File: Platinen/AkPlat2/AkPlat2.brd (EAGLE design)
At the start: 61.8 x 50.4 mm, 16 parts, among them CON1 XT30UPB-M

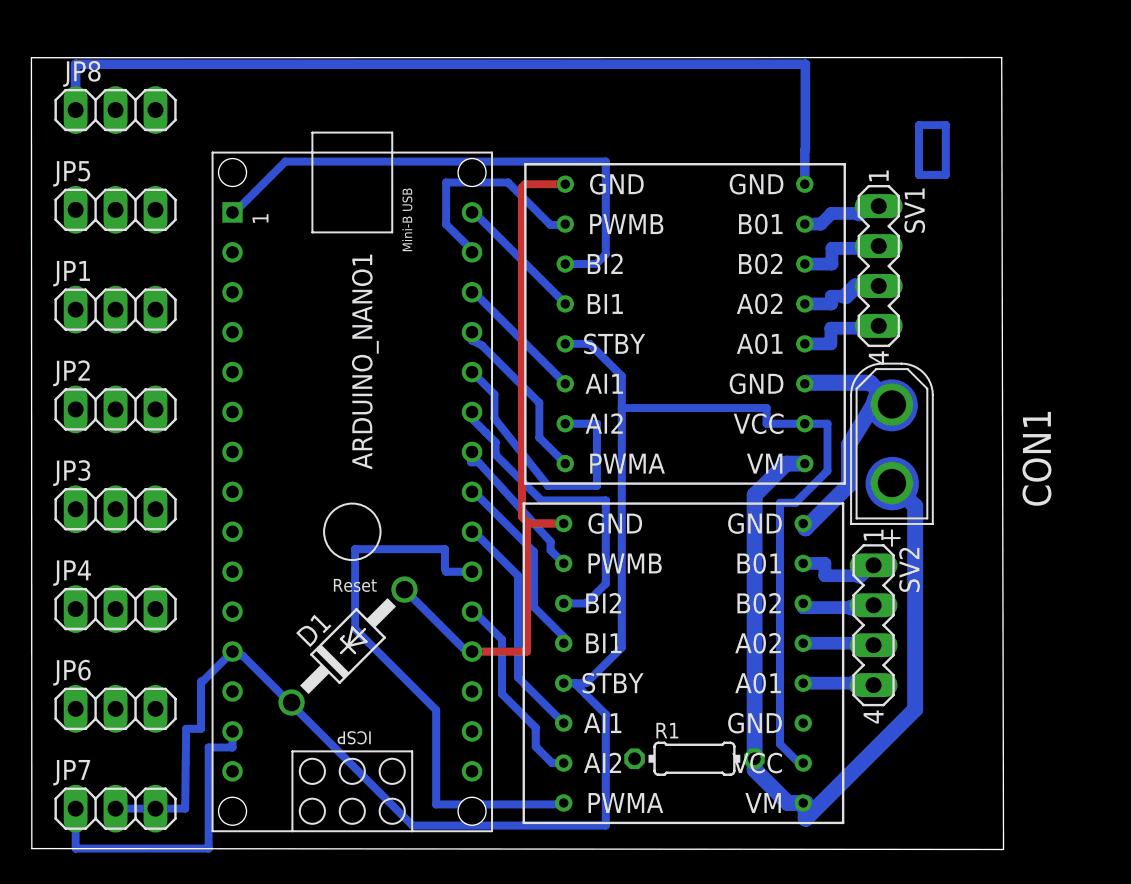
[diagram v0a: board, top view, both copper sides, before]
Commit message: PCB almost done
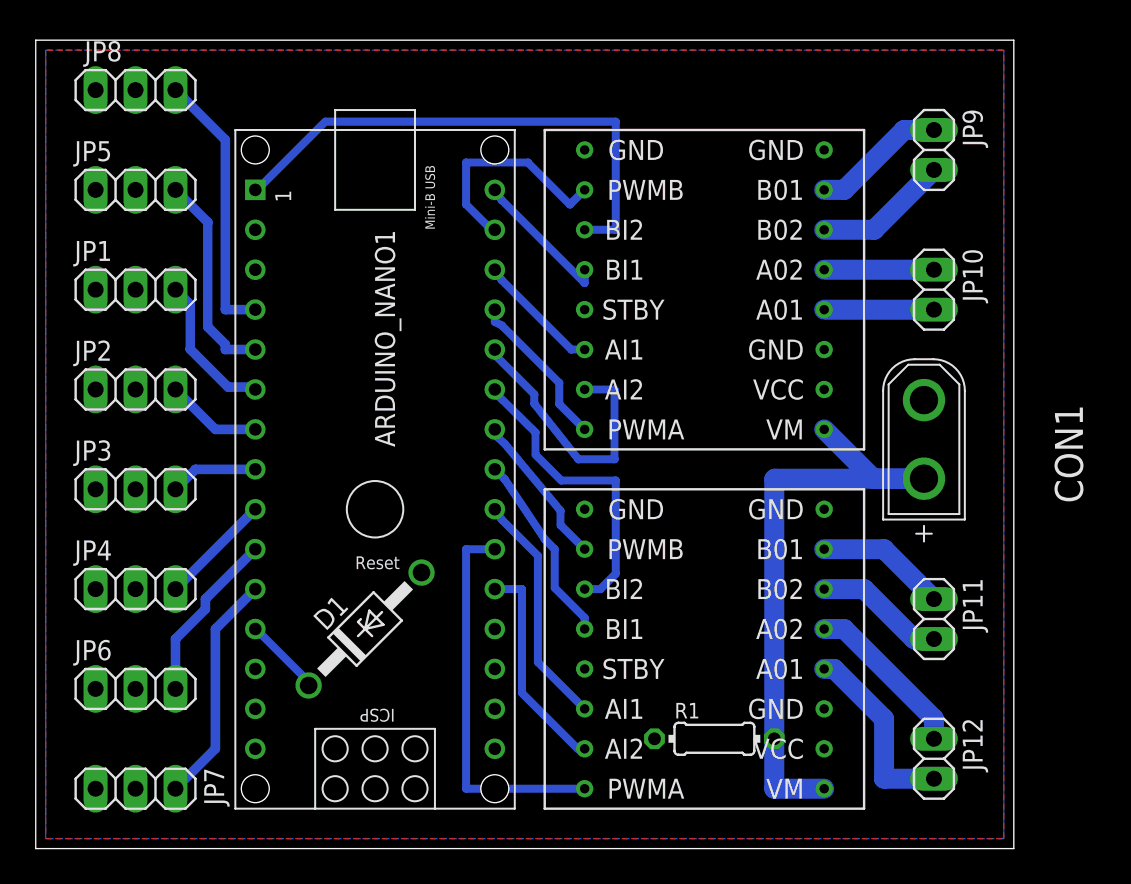
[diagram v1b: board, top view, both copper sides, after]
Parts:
- removed SV1, SV2: (no value), con-lstb:MA04-1
- added JP10, JP11, JP12, JP9: (no value), pinhead:1X02
- moved U$1 2.50 mm to (52.7, 45.7)
- moved CON1 2.06 mm to (56.5, 26.0)
- moved ARDUINO_NANO1 2.04 mm to (21.6, 21.6)
- moved R1 1.80 mm to (43.2, 6.99)
- moved JP1 1.80 mm to (6.35, 35.6)
- moved JP4 1.80 mm to (6.35, 16.5)
- moved JP7 1.80 mm to (6.35, 3.81)
- moved JP2 1.80 mm to (6.35, 29.2)
- moved JP3 1.80 mm to (6.35, 22.9)
- moved JP6 1.80 mm to (6.35, 10.2)
- moved JP5 1.80 mm to (6.35, 41.9)
- moved JP8 1.80 mm to (6.35, 48.3)
- moved U$2 1.61 mm to (52.7, 22.9)
- moved D1 1.53 mm to (21.0, 14.0)
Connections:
- net N$28 renamed 5V
- net N$8 renamed VM
- removed net N$1: ARDUINO_NANO1.19, D1.A, U$1.9, U$2.9
- removed net N$15: ARDUINO_NANO1.14, JP1.1, JP2.1, JP3.1, JP4.1, JP5.1, JP6.1, JP7.1, JP8.1, U$1.1
- removed net N$2: CON1.-, U$1.6, U$2.1
- new net GND: ARDUINO_NANO1.14, ARDUINO_NANO1.19, CON1.-, D1.A, JP1.1, JP2.1, JP3.1, JP4.1, JP5.1, JP6.1, JP7.1, JP8.1, U$1.1, U$1.6, U$1.9, U$2.1, U$2.6, U$2.9
- net N$16: now also JP9.1; no longer SV1.1
- net N$17: now also JP9.2; no longer SV1.2
- net N$18: now also JP10.1; no longer SV1.3
- net N$19: now also JP10.2; no longer SV1.4
- net N$20: now also JP11.1; no longer SV2.1
- net N$21: now also JP11.2; no longer SV2.2
- net N$22: now also JP12.1; no longer SV2.3
- net N$23: now also JP12.2; no longer SV2.4
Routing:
- net 5V: track 120.3 -> 5.01 mm
- net N$15: track 77.0 -> 0.00 mm
- net N$1: track 44.3 -> 0.00 mm
- net N$35: track 0.00 -> 17.2 mm
- net N$2: track 17.1 -> 0.00 mm
- net N$26: track 0.00 -> 14.8 mm
- net N$34: track 0.00 -> 13.4 mm
- net VM: track 51.7 -> 40.1 mm
- net N$27: track 0.00 -> 11.0 mm
- net N$11: track 35.4 -> 24.6 mm
- net N$29: track 9.75 -> 0.00 mm
- net N$33: track 0.00 -> 9.38 mm
- net N$23: track 4.88 -> 12.1 mm
- net N$30: track 0.00 -> 7.18 mm
- net N$32: track 0.00 -> 6.13 mm
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- added copper zone on layer 16, net 5V
- added copper zone on layer 1, net GND
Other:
- board size 61.8 x 50.4 mm -> 62.2 x 51.4 mm

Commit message: PCB fertig Gerber fertig
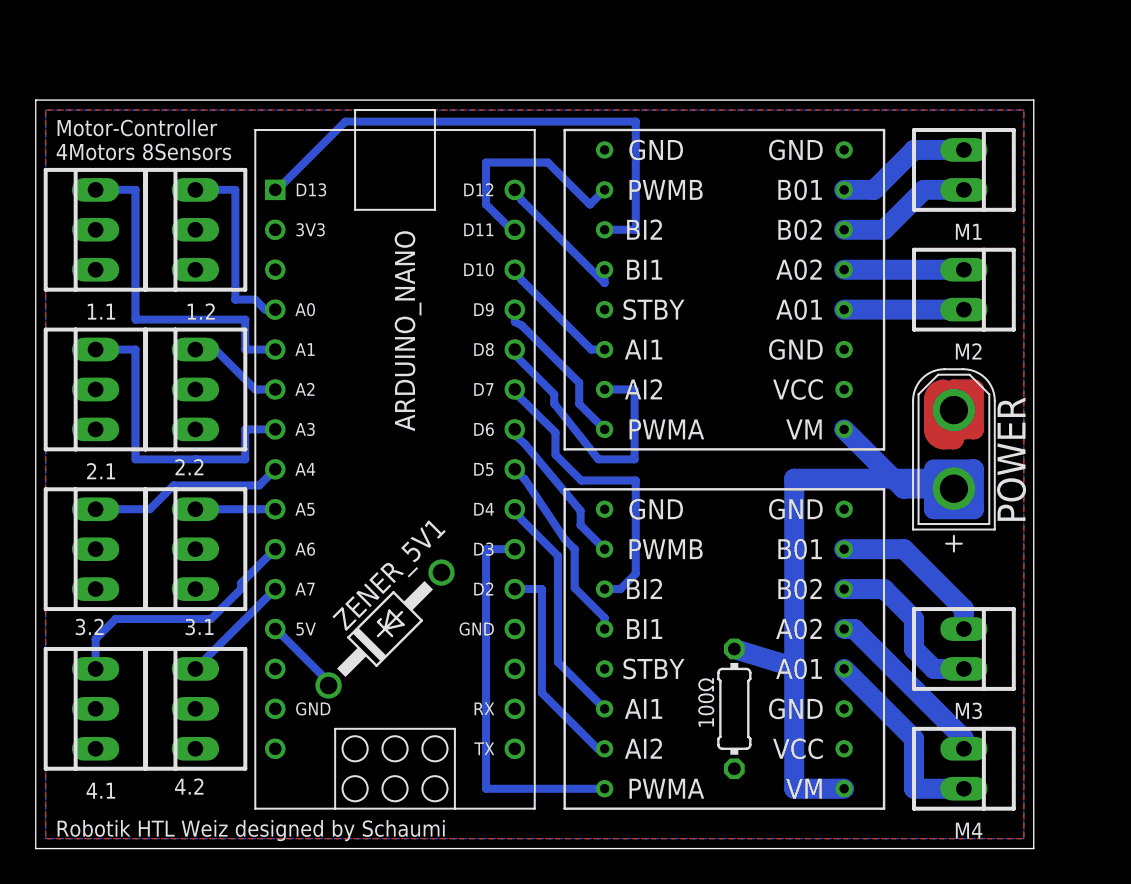
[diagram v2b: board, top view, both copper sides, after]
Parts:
- removed ARDUINO_NANO1: (no value), ArduinoNanoV30:ARDUINO_NANO
- removed CON1: XT30UPB-M, amass:XT30UPB-M
- removed D1: BZX85, diode:DO41Z10
- removed JP1, JP2, JP3, JP4, JP5, JP6, JP7, JP8: (no value), pinhead:1X03
- removed JP10, JP11, JP12, JP9: (no value), pinhead:1X02
- removed R1: (no value), rcl:0204/7
- added 1.1, 1.2, 2.1, 2.2, 3.1, 3.2, 4.1, 4.2: 22-23-2031, con-molex:22-23-2031
- added 100Ω: 100, rcl:0204/7
- added ARDUINO_NANO: (no value), ArduinoNanoV30:ARDUINO_NANO
- added M1, M2, M3, M4: 22-23-2021, con-molex:22-23-2021
- added POWER: XT30UPB-M, amass:XT30UPB-M
- added ZENER_5V1: BZX85, diode:DO41Z10
- moved U$1 1.27 mm to (54.0, 45.7)
- moved U$2 1.27 mm to (54.0, 22.9)
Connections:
- net 5V: now also 1.1.2, 1.2.2, 100Ω.1, 2.1.2, 2.2.2, 3.1.2, 3.2.2, 4.1.2, 4.2.2, ARDUINO_NANO.12, ZENER_5V1.C; no longer ARDUINO_NANO1.12, D1.C, JP1.2, JP2.2, JP3.2, JP4.2, JP5.2, JP6.2, JP7.2, JP8.2, R1.1
- net BIN2: now also ARDUINO_NANO.1; no longer ARDUINO_NANO1.1
- net GND: now also 1.1.1, 1.2.1, 2.1.1, 2.2.1, 3.1.1, 3.2.1, 4.1.1, 4.2.1, ARDUINO_NANO.14, ARDUINO_NANO.19, POWER.-, ZENER_5V1.A; no longer ARDUINO_NANO1.14, ARDUINO_NANO1.19, CON1.-, D1.A, JP1.1, JP2.1, JP3.1, JP4.1, JP5.1, JP6.1, JP7.1, JP8.1
- net N$10: now also ARDUINO_NANO.24; no longer ARDUINO_NANO1.24
- net N$11: now also ARDUINO_NANO.21; no longer ARDUINO_NANO1.21
- net N$12: now also ARDUINO_NANO.20; no longer ARDUINO_NANO1.20
- net N$13: now also ARDUINO_NANO.22; no longer ARDUINO_NANO1.22
- net N$14: now also ARDUINO_NANO.23; no longer ARDUINO_NANO1.23
- net N$16: now also M1.1; no longer JP9.1
- net N$17: now also M1.2; no longer JP9.2
- net N$18: now also M2.1; no longer JP10.1
- net N$19: now also M2.2; no longer JP10.2
- net N$20: now also M3.1; no longer JP11.1
- net N$21: now also M3.2; no longer JP11.2
- net N$22: now also M4.1; no longer JP12.1
- net N$23: now also M4.2; no longer JP12.2
- net N$26: now also 4.2.3, ARDUINO_NANO.11; no longer ARDUINO_NANO1.11, JP7.3
- net N$27: now also 4.1.3, ARDUINO_NANO.10; no longer ARDUINO_NANO1.10, JP6.3
- net N$3: now also ARDUINO_NANO.27; no longer ARDUINO_NANO1.27
- net N$30: now also 3.1.3, ARDUINO_NANO.9; no longer ARDUINO_NANO1.9, JP4.3
- net N$31: now also 3.2.3, ARDUINO_NANO.8; no longer ARDUINO_NANO1.8, JP3.3
- net N$32: now also 2.1.3, ARDUINO_NANO.7; no longer ARDUINO_NANO1.7, JP2.3
- net N$33: now also 2.2.3, ARDUINO_NANO.6; no longer ARDUINO_NANO1.6, JP1.3
- net N$34: now also 1.1.3, ARDUINO_NANO.5; no longer ARDUINO_NANO1.5, JP5.3
- net N$35: now also 1.2.3, ARDUINO_NANO.4; no longer ARDUINO_NANO1.4, JP8.3
- net N$4: now also ARDUINO_NANO.25; no longer ARDUINO_NANO1.25
- net N$5: now also ARDUINO_NANO.30; no longer ARDUINO_NANO1.30
- net N$6: now also ARDUINO_NANO.29; no longer ARDUINO_NANO1.29
- net N$7: now also ARDUINO_NANO.28; no longer ARDUINO_NANO1.28
- net N$9: now also ARDUINO_NANO.26; no longer ARDUINO_NANO1.26
- net VIN: now also ARDUINO_NANO.15; no longer ARDUINO_NANO1.15
- net VM: now also 100Ω.2, POWER.+; no longer CON1.+, R1.2
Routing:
- net VM: track 40.1 -> 54.8 mm
- net N$32: track 6.13 -> 20.3 mm
- net GND: track 0.00 -> 11.0 mm
- net N$34: track 13.4 -> 21.6 mm
- net N$26: track 14.8 -> 7.18 mm
- net N$31: track 5.61 -> 12.5 mm
- net N$27: track 11.0 -> 15.9 mm
- net N$35: track 17.2 -> 12.3 mm
- net N$33: track 9.38 -> 6.13 mm
- net N$21: track 8.30 -> 10.8 mm
- net N$20: track 8.30 -> 10.5 mm
- net N$30: track 7.18 -> 5.08 mm
- net N$19: track 6.98 -> 7.62 mm
- net N$18: track 6.98 -> 7.62 mm
- net N$23: track 12.1 -> 12.6 mm
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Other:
- board size 62.2 x 51.4 mm -> 63.5 x 47.6 mm
- board text added: "+"
- board text added: "GND"
- board text added: "Motor-Controller 4Motors 8Sensors"
- board text added: "Robotik HTL Weiz designed by Schaumi"
- board text added: "S + -"
- board text added: "VCC"
